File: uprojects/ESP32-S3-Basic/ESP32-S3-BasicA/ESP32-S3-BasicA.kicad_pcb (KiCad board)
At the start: 2 copper layers, 11 parts, among them J1 USB_C_Receptacle, U1 ESP32-S3-WROOM-1x-N8R8, U2 CH340G, Y2 12MHz

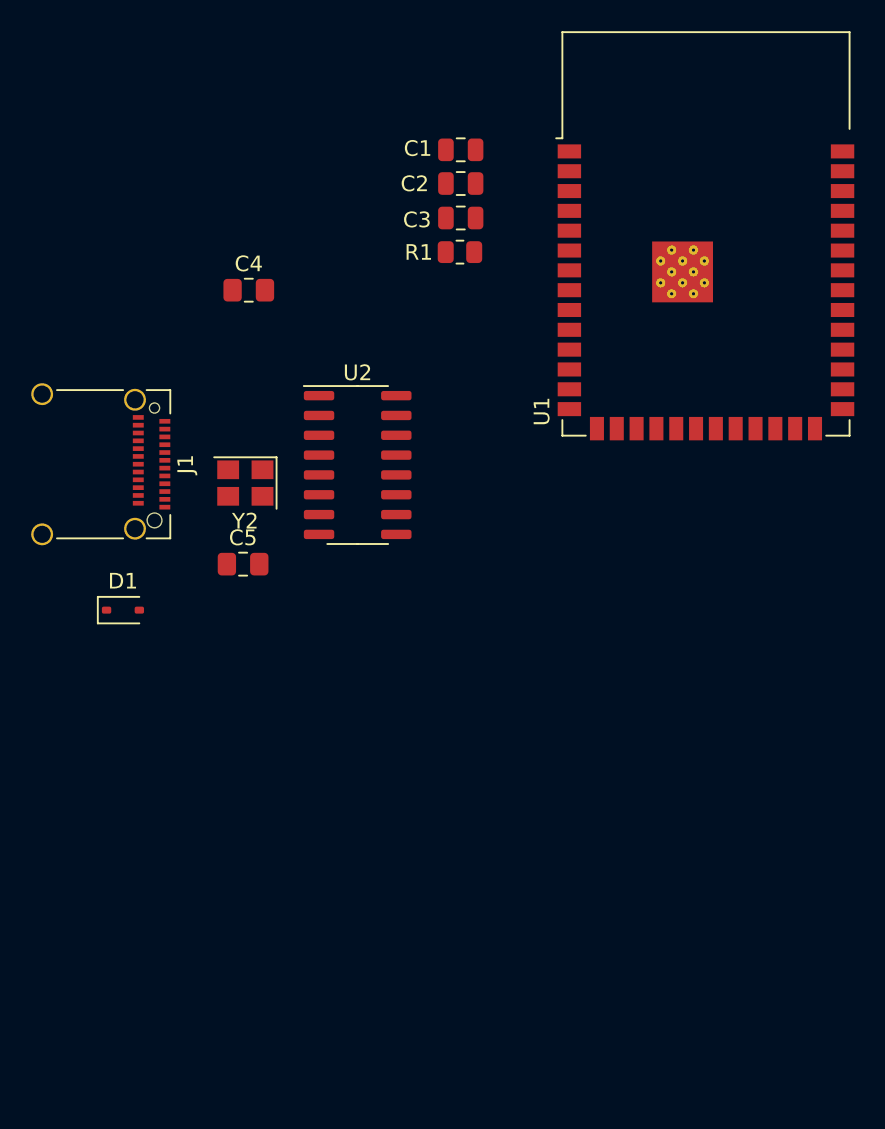
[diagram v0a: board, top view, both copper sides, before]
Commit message: April 2 commit
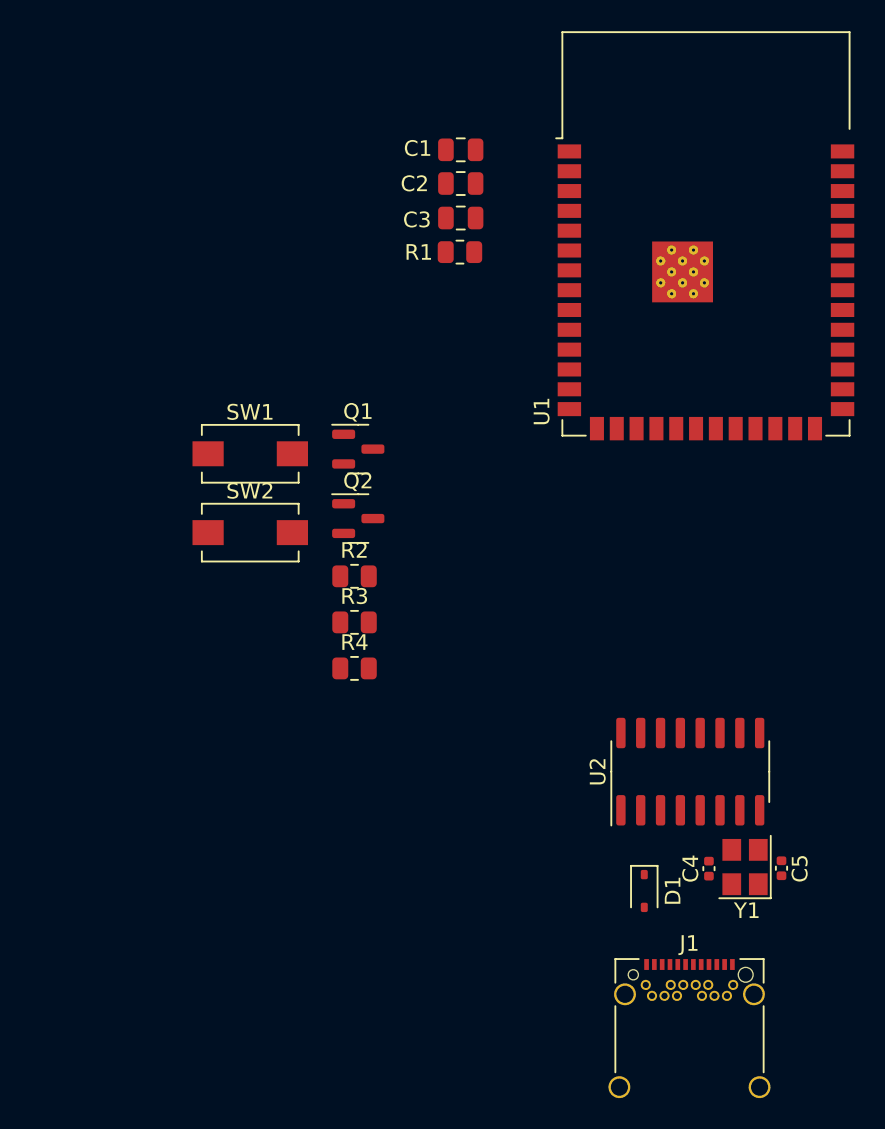
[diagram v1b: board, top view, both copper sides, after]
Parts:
- removed Y2: 12MHz, Crystal:Crystal_SMD_3225-4Pin_3.2x2.5mm
- added Q1: BC817, Package_TO_SOT_SMD:SOT-23, F.Cu at (128.4, 78.1)
- added Q2: BC817, Package_TO_SOT_SMD:SOT-23, F.Cu at (128.4, 82.5)
- added R2: 4k7/R0402, Resistor_SMD:R_0805_2012Metric, F.Cu at (128.1, 86.2)
- added R3: 4k7/R0402, Resistor_SMD:R_0805_2012Metric, F.Cu at (128.1, 89.2)
- added R4: 4k7/R0402, Resistor_SMD:R_0805_2012Metric, F.Cu at (128.1, 92.1)
- added SW1: ESP32_EN, Button_Switch_SMD:SW_SPST_EVQPE1, F.Cu at (121.4, 78.4)
- added SW2: ESP32_EN, Button_Switch_SMD:SW_SPST_EVQPE1, F.Cu at (121.4, 83.4)
- added Y1: 12MHz, Crystal:Crystal_SMD_3225-4Pin_3.2x2.5mm, F.Cu at (153.1, 104.9)
- C4, C5: footprint Capacitor_SMD:C_0805_2012Metric_Pad1.18x1.45mm_HandSolder -> Capacitor_SMD:C_0402_1005Metric
- J1: footprint Connector_USB:USB_C_Receptacle_Amphenol_12401610E4-2A_CircularHoles -> Connector_USB:USB_C_Receptacle_Amphenol_12401548E4-2A_CircularHoles
- moved J1 53.5 mm to (149.6, 116.1), turned to 0 degrees
- moved C4 47.4 mm to (150.8, 105.0), turned to 90 degrees
- moved C5 39.6 mm to (155.5, 104.9), turned to 90 degrees
- moved D1 37.9 mm to (146.7, 106.4), turned to -90 degrees
- moved U2 29.0 mm to (149.6, 98.7), turned to 90 degrees
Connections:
- U1 pad 27: unconnected-(U1-IO0/RTC_GPIO0/GPIO0-Pad27) -> GPIO00\BUT1
- U2 pad 13: unconnected-(U2-~{DTR}-Pad13) -> Net-(Q2-E)
- U2 pad 14: unconnected-(U2-~{RTS}-Pad14) -> Net-(Q1-E)
- U2 pad 9: unconnected-(U2-~{CTS}-Pad9) -> Net-(U2-~{CTS})
